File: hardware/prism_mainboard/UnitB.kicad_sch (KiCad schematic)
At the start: 1 part, among them U1 XC7Z015-2CLG485I

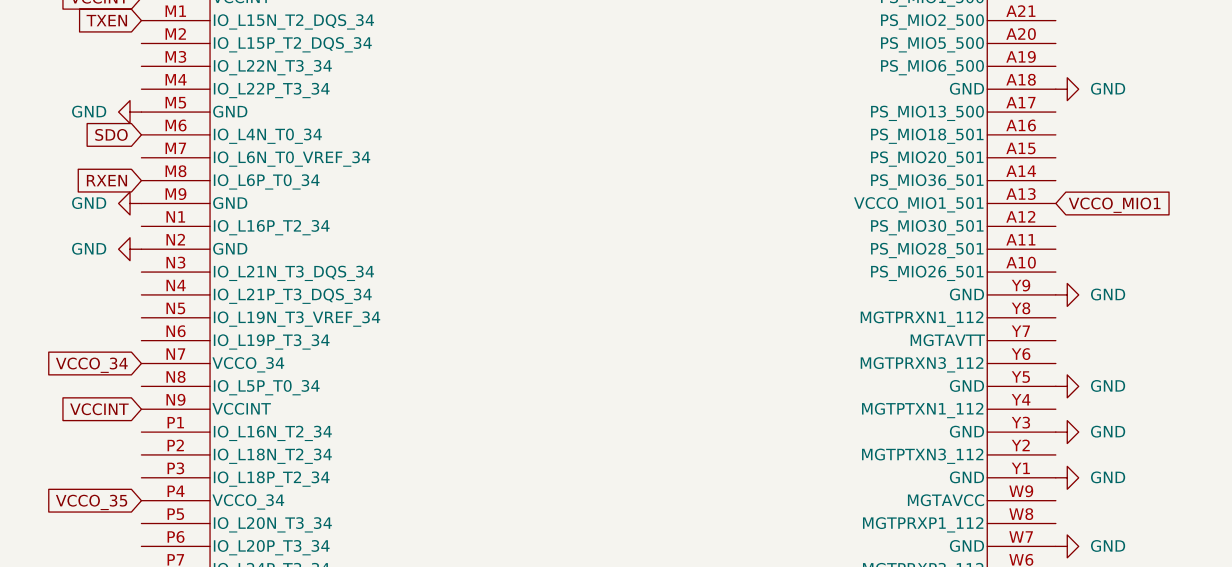
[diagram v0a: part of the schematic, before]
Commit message: Updates
Mostly Schematic updates, nothing too big. Added a few datasheets
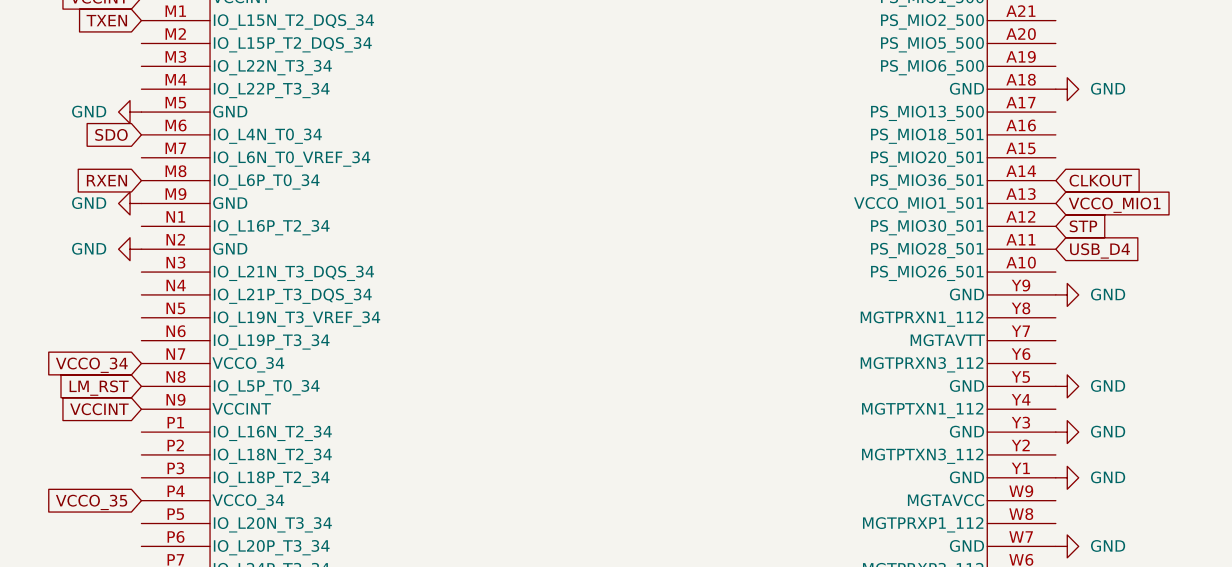
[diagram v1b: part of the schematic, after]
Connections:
- net USB_D4: now reaches U1.A11 (PS_MIO28_501)
- net STP: now reaches U1.A12 (PS_MIO30_501)
- net CLKOUT: now reaches U1.A14 (PS_MIO36_501)
- net LM_RST: now reaches U1.N8 (IO_L5P_T0_34)
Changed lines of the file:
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@@
+		)
+	)
+	(global_label "LM_RST"
+		(shape input)
+		(at 99.06 78.74 180)
+		(fields_autoplaced yes)
+		(effects
+			(font
+				(size 1.27 1.27)
+			)
+			(justify right)
+		)
+		(property "Intersheetrefs" "${INTERSHEET_REFS}"
+			(at 89.1806 78.74 0)
+			(hide yes)
+			(show_name no)
+			(do_not_autoplace no)
+			(effects
+				(font
+					(size 1.27 1.27)
+				)
+				(justify right)
+			)
 		)
 	)
@@
 		)
 	)
+	(global_label "USB_D4"
+		(shape input)
+		(at 200.66 63.5 0)
+		(fields_autoplaced yes)
+		(effects
+			(font
+				(size 1.27 1.27)
+			)
+			(justify left)
+		)
+		(property "Intersheetrefs" "${INTERSHEET_REFS}"
+			(at 210.9023 63.5 0)
+			(hide yes)
+			(show_name no)
+			(do_not_autoplace no)
+			(effects
+				(font
+					(size 1.27 1.27)
+				)
+				(justify left)
+			)
+		)
+	)
 	(global_label "SDO"
 		(shape input)
@@
 		)
 	)
+	(global_label "CLKOUT"
+		(shape input)
+		(at 200.66 55.88 0)
+		(fields_autoplaced yes)
+		(effects
+			(font
+				(size 1.27 1.27)
+			)
+			(justify left)
+		)
+		(property "Intersheetrefs" "${INTERSHEET_REFS}"
+			(at 210.8419 55.88 0)
+			(hide yes)
+			(show_name no)
+			(do_not_autoplace no)
+			(effects
+				(font
+					(size 1.27 1.27)
+				)
+				(justify left)
+			)
+		)
+	)
 	(global_label "TXEN"
 		(shape input)
@@
 			)
 		)
+	)
+	(global_label "STP"
+		(shape input)
+		(at 200.66 60.96 0)
+		(fields_autoplaced yes)
+		(effects
+			(font
+				(size 1.27 1.27)
+			)
+			(justify left)
+		)
+		(property "Intersheetrefs" "${INTERSHEET_REFS}"
+			(at 207.0923 60.96 0)
+			(hide yes)
+			(show_name no)
+			(do_not_autoplace no)
+			(effects
+				(font
+					(size 1.27 1.27)
+				)
+				(justify left)
+			)
+		)
